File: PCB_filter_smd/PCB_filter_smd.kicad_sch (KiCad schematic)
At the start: 24 parts, among them J2 Conn_01x02_Pin, U1 AD620, U2 LM324

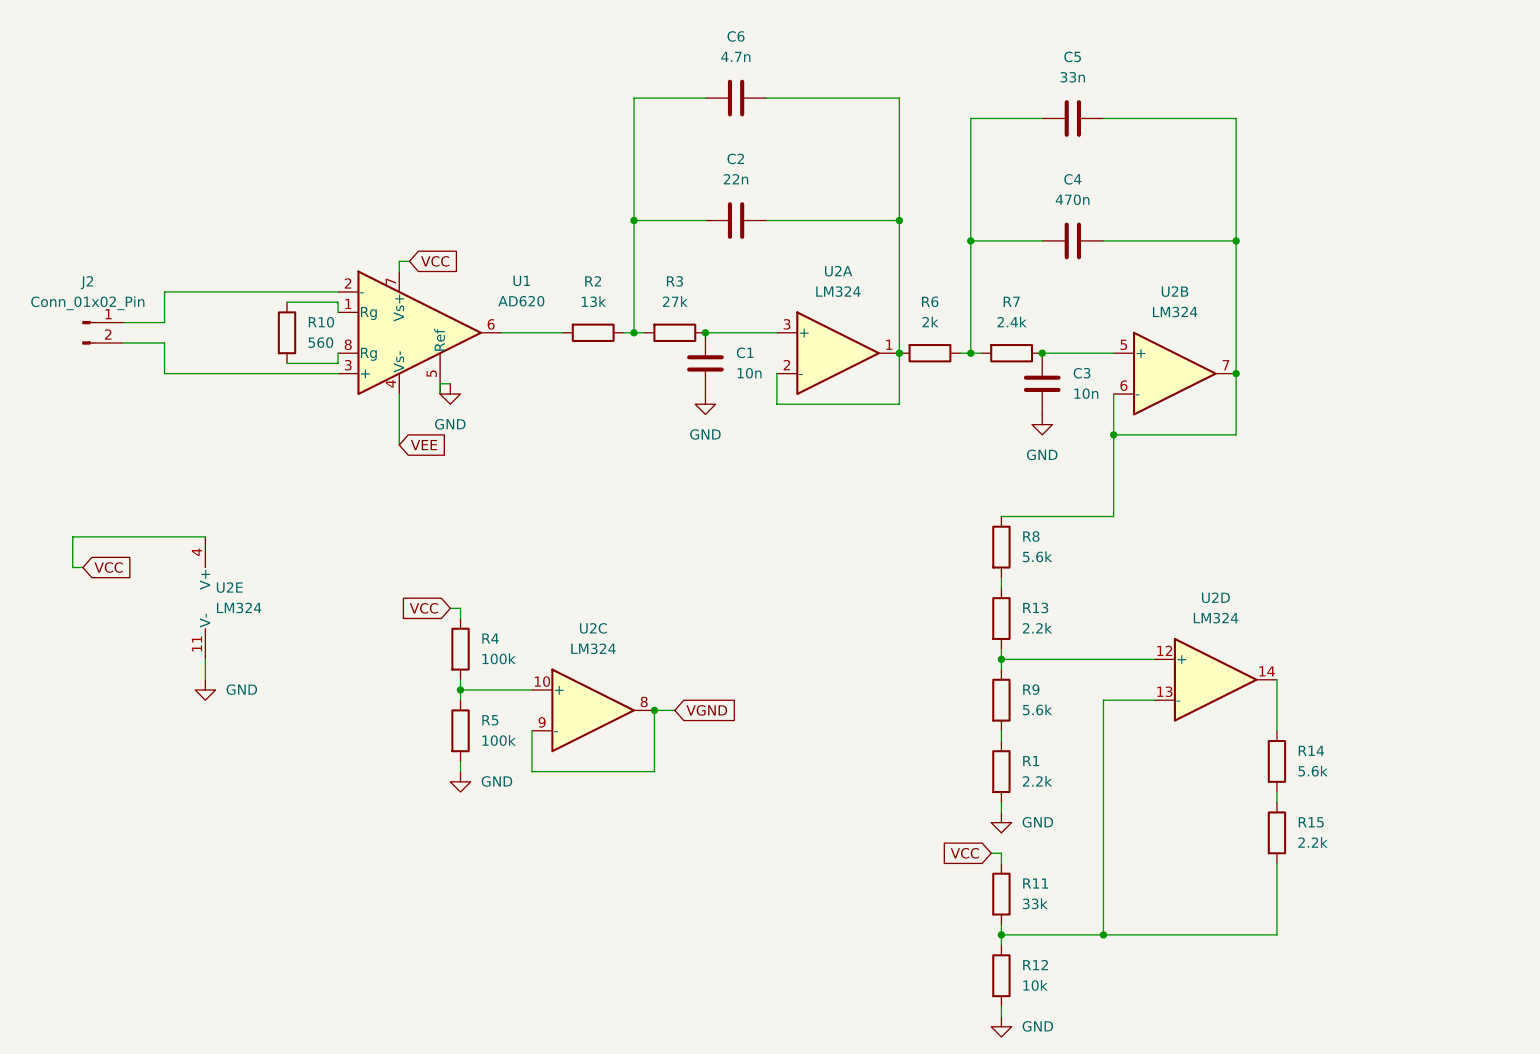
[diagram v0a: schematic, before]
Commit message: last
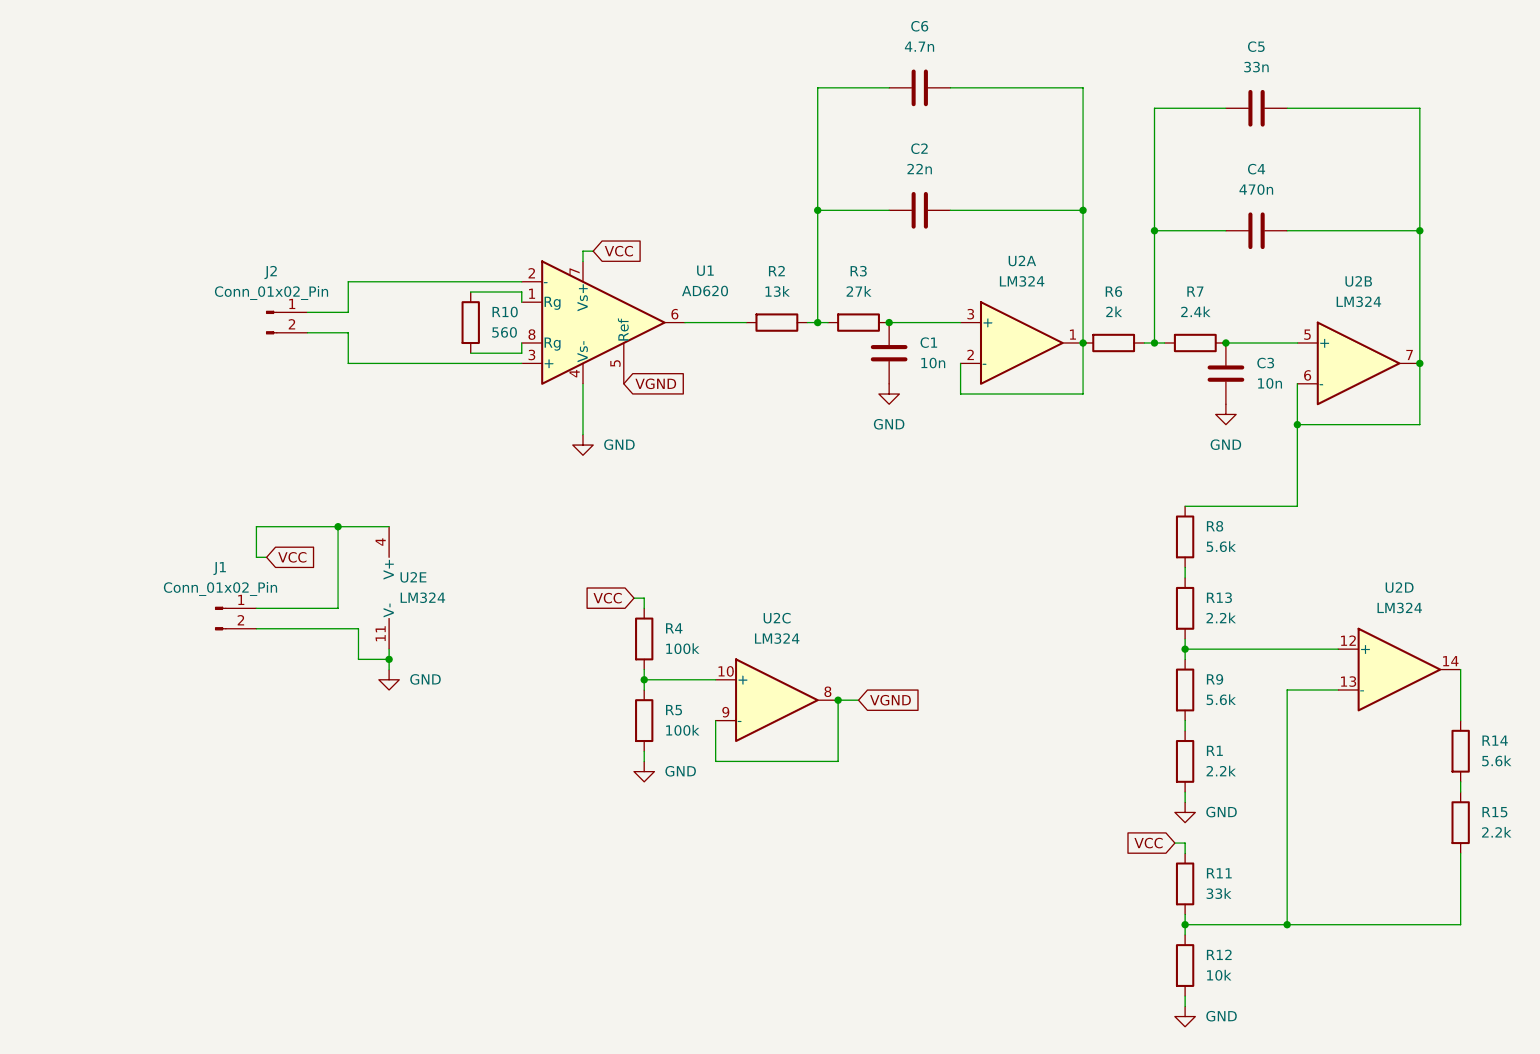
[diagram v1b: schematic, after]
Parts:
- added J1: Conn_01x02_Pin, Connector_PinHeader_2.54mm:PinHeader_1x02_P2.54mm_Vertical, symbol Connector:Conn_01x02_Pin
- C3: footprint Capacitor_THT:C_Disc_D5.0mm_W2.5mm_P2.50mm -> Capacitor_SMD:C_0805_2012Metric_Pad1.18x1.45mm_HandSolder
- R10, R6, R7: footprint Resistor_THT:R_Axial_DIN0207_L6.3mm_D2.5mm_P7.62mm_Horizontal -> Resistor_SMD:R_0805_2012Metric_Pad1.20x1.40mm_HandSolder
- U2: footprint (none) -> Package_SO:SOIC-14_3.9x8.7mm_P1.27mm
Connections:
- net VEE is gone; now on net GND: U1.4 (Vs-)
- net GND: now also J1.2 (Pin_2); no longer U1.5 (Ref)
- net VCC: now also J1.1 (Pin_1)
- net VGND: now also U1.5 (Ref)
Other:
- moved on the sheet: C1, C2, C3, C4, C5, C6, J2, R1, R10, R11, R12, R13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
